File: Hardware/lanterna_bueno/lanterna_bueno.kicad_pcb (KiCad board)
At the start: 2 copper layers, 75.1 x 56.5 mm, 51 parts, among them P1 USB_C_Plug_USB2.0, Q1 BC807, Q2 2SK4075, Q3 2SK4075, Q4 2SK4075, Q5 2SK4075, SW1 SW_Push, SW2 SW_Push, SW3 SW_Push, U1 RT9193-33, U2 IR2101, U3 IR2101, U4 STM32F042K6Tx, U5 TP4056

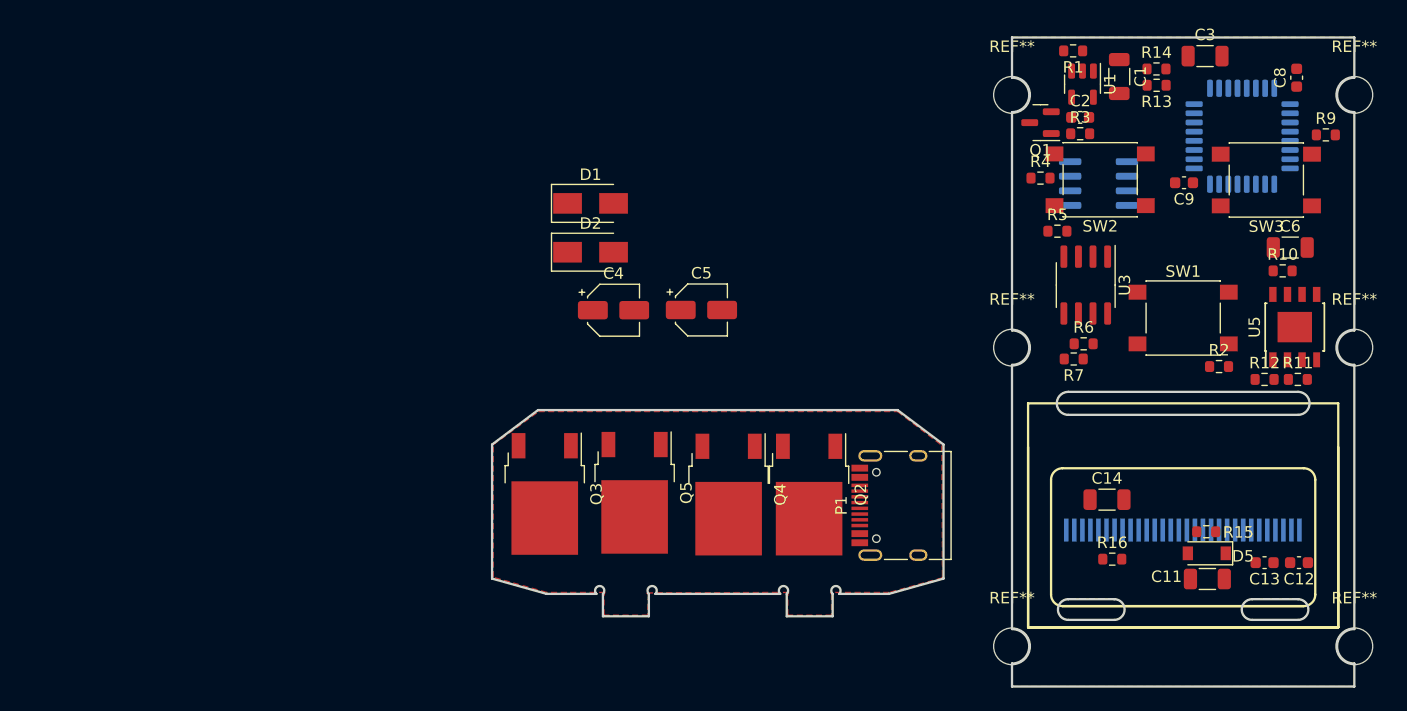
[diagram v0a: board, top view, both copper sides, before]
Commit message: building pcb
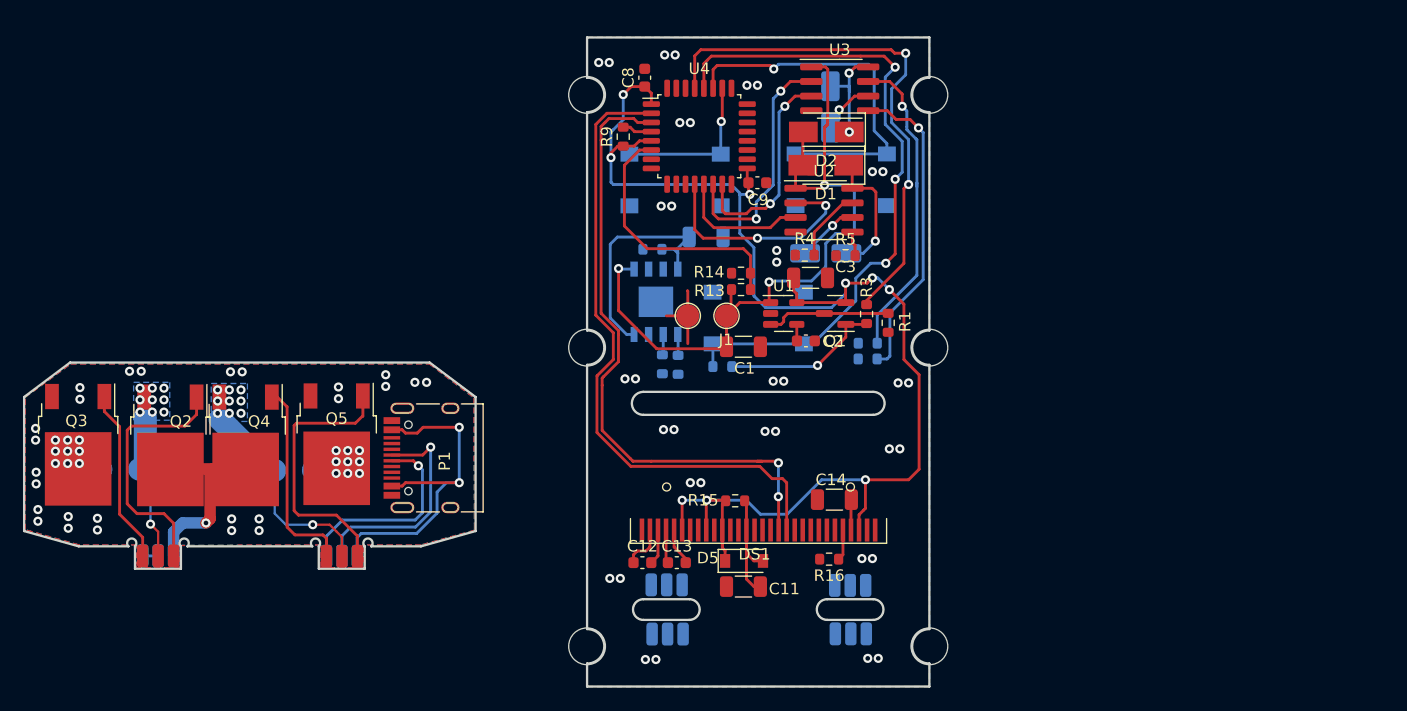
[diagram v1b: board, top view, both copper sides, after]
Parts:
- added J1: Conn_01x02_Male, Connector:SMD_BAT, F.Cu at (147.8, 92.4)
- added J10: Conn_01x03_Male, Connector:3pin 90 pcb solder, B.Cu at (160.2, 113.1)
- added J11: Conn_01x03_Male, Connector:3pin 90 pcb solder, B.Cu at (157.1, 122.8)
- added J2: Conn_01x02_Male, Connector:SMD_BAT, B.Cu at (96.8, 105.7)
- added J3: Conn_01x02_Male, Connector:SMD_BAT, B.Cu at (108.5, 105.8)
- added J4: Conn_01x03_Male, Connector:3pin 90 pcb solder, B.Cu at (112.8, 116.0)
- added J5: Conn_01x03_Male, Connector:3pin 90 pcb solder, B.Cu at (96.8, 116.0)
- added J6: Conn_01x03_Male, Connector:3pin 90 pcb solder, F.Cu at (96.8, 110.5)
- added J7: Conn_01x03_Male, Connector:3pin 90 pcb solder, F.Cu at (116.0, 116.1)
- added J8: Conn_01x03_Male, Connector:3pin 90 pcb solder, B.Cu at (141.0, 118.5)
- added J9: Conn_01x03_Male, Connector:3pin 90 pcb solder, B.Cu at (141.1, 122.8)
- C4, C5, C6, R10, R11, R12, R2, R6, R7, REF** (x6), SW1, SW2, SW3, U5: moved to B.Cu
- DS1, U2, U4: moved to F.Cu
- moved REF** 66.8 mm to (135.7, 121.1), turned to 180 degrees
- moved REF** 66.8 mm to (135.7, 95.1), turned to 180 degrees
- moved REF** 66.8 mm to (135.7, 73.1), turned to 180 degrees
- moved R9 61.2 mm to (138.9, 76.8), turned to 90 degrees
- moved C12 57.2 mm to (140.5, 113.9), turned to 0 degrees
- moved C8 56.8 mm to (140.7, 71.6)
- moved Q2 55.8 mm to (99.4, 103.6)
- moved U5 55.7 mm to (141.7, 91.2)
- moved R11 55.3 mm to (142.3, 96.6), turned to -90 degrees
- moved R10 54.9 mm to (141.4, 86.6), turned to 180 degrees
- moved SW3 51.5 mm to (143.4, 80.6), turned to 0 degrees
- moved C13 51.2 mm to (143.5, 113.9), turned to 0 degrees
- moved R12 51.1 mm to (143.6, 96.6), turned to -90 degrees
- moved C6 50.9 mm to (146.1, 85.5)
- moved U4 47.3 mm to (145.5, 76.7), turned to 0 degrees
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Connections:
- C4 pad 2: Net-(C4-Pad2) -> TRANSISTOR_1_P2_1
- C5 pad 2: Net-(C5-Pad2) -> TRANSISTOR_2_P2_1
- P1 pad A1: GND -> GND_2
- P1 pad A12: GND -> GND_2
- P1 pad A4: Net-(R10-Pad2) -> VBUS_2
- P1 pad A6: unconnected-(P1-PadA6) -> DP_2
- P1 pad A7: unconnected-(P1-PadA7) -> DM_2
- P1 pad A9: Net-(R10-Pad2) -> VBUS_2
- P1 pad B1: GND -> GND_2
- P1 pad B12: GND -> GND_2
- P1 pad B4: Net-(R10-Pad2) -> VBUS_2
- P1 pad B9: Net-(R10-Pad2) -> VBUS_2
- P1 pad S1: GND -> GND_2
- Q2 pad 1: Net-(Q2-Pad1) -> TRANSISTOR_1_P1_2
- Q2 pad 2: BATT -> BATT_2
- Q2 pad 3: Net-(C4-Pad2) -> LED_SUP+
- Q3 pad 1: Net-(Q3-Pad1) -> TRANSISTOR_1_P3_2
- Q3 pad 2: Net-(D3-Pad1) -> LED_SUP-
- Q3 pad 3: GND -> GND_2
- Q4 pad 1: Net-(Q4-Pad1) -> TRANSISTOR_2_P1_2
- Q4 pad 2: BATT -> BATT_2
- Q4 pad 3: Net-(C5-Pad2) -> LED_INF+
- Q5 pad 1: Net-(Q5-Pad1) -> TRANSISTOR_2_P3_2
- Q5 pad 2: Net-(D4-Pad1) -> LED_INF-
- Q5 pad 3: GND -> GND_2
- R10 pad 2: Net-(R10-Pad2) -> VBUS_1
- R4 pad 1: Net-(Q2-Pad1) -> TRANSISTOR_1_P1_1
- R5 pad 1: Net-(Q3-Pad1) -> TRANSISTOR_1_P3_1
- R6 pad 1: Net-(Q4-Pad1) -> TRANSISTOR_2_P1_1
- R7 pad 1: Net-(Q5-Pad1) -> TRANSISTOR_2_P3_1
- U2 pad 6: Net-(C4-Pad2) -> TRANSISTOR_1_P2_1
- U3 pad 6: Net-(C5-Pad2) -> TRANSISTOR_2_P2_1
- U4 pad 21: unconnected-(U4-Pad21) -> DM_1
- U4 pad 22: unconnected-(U4-Pad22) -> DP_1
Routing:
- net +3V3: track 0.00 -> 120.8 mm, vias 0 -> 9
- net BATT: track 0.00 -> 64.8 mm, vias 0 -> 3
- net BUT_MENU: track 0.00 -> 59.2 mm, vias 0 -> 3
- net LCD_SDA: track 0.00 -> 55.7 mm
- net LCD_SCL: track 0.00 -> 55.2 mm, vias 0 -> 2
- net POWER_CMD: track 0.00 -> 46.1 mm, vias 0 -> 2
- net BUT_PLUS: track 0.00 -> 32.0 mm, vias 0 -> 1
- net VBUS_2: track 0.00 -> 30.6 mm, vias 0 -> 2
- net Net-(R7-Pad2): track 0.00 -> 27.5 mm, vias 0 -> 1
- net Net-(R6-Pad2): track 0.00 -> 27.4 mm, vias 0 -> 1
- net TRANSISTOR_2_P3_2: track 0.00 -> 23.7 mm
- net BAT_MON: track 0.00 -> 23.2 mm
- net TRANSISTOR_1_P1_2: track 0.00 -> 22.1 mm
- net PWM_LED_INFH: track 0.00 -> 21.5 mm, vias 0 -> 2
- net Net-(C6-Pad1): track 0.00 -> 20.9 mm
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- added copper zone on B.Cu, net GND_2
- added copper zone on F.Cu, net GND_2
- added copper zone on B.Cu, net LED_INF+
- added copper zone on B.Cu, net LED_INF-
- added copper zone on B.Cu, net LED_SUP+
- added copper zone on B.Cu, net LED_SUP-
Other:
- board size 75.1 x 56.5 mm -> 78.8 x 56.5 mm
